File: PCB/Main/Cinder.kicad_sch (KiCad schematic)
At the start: 22 parts, among them J1 Heater -, J2 Heater +, J3 Fan +, J4 Fan -, Q1 IPD33CN10N G, Q2 IPD33CN10N G, SW1 SW_Push, SW2 SW_Push, SW3 SW_Push, SW9 EC11E09244BS, U1 RP2040-ZERO, U2 HS96L03W2C03, U3 XT60PW-F_C428722, U4 K7805-500R3_C909662

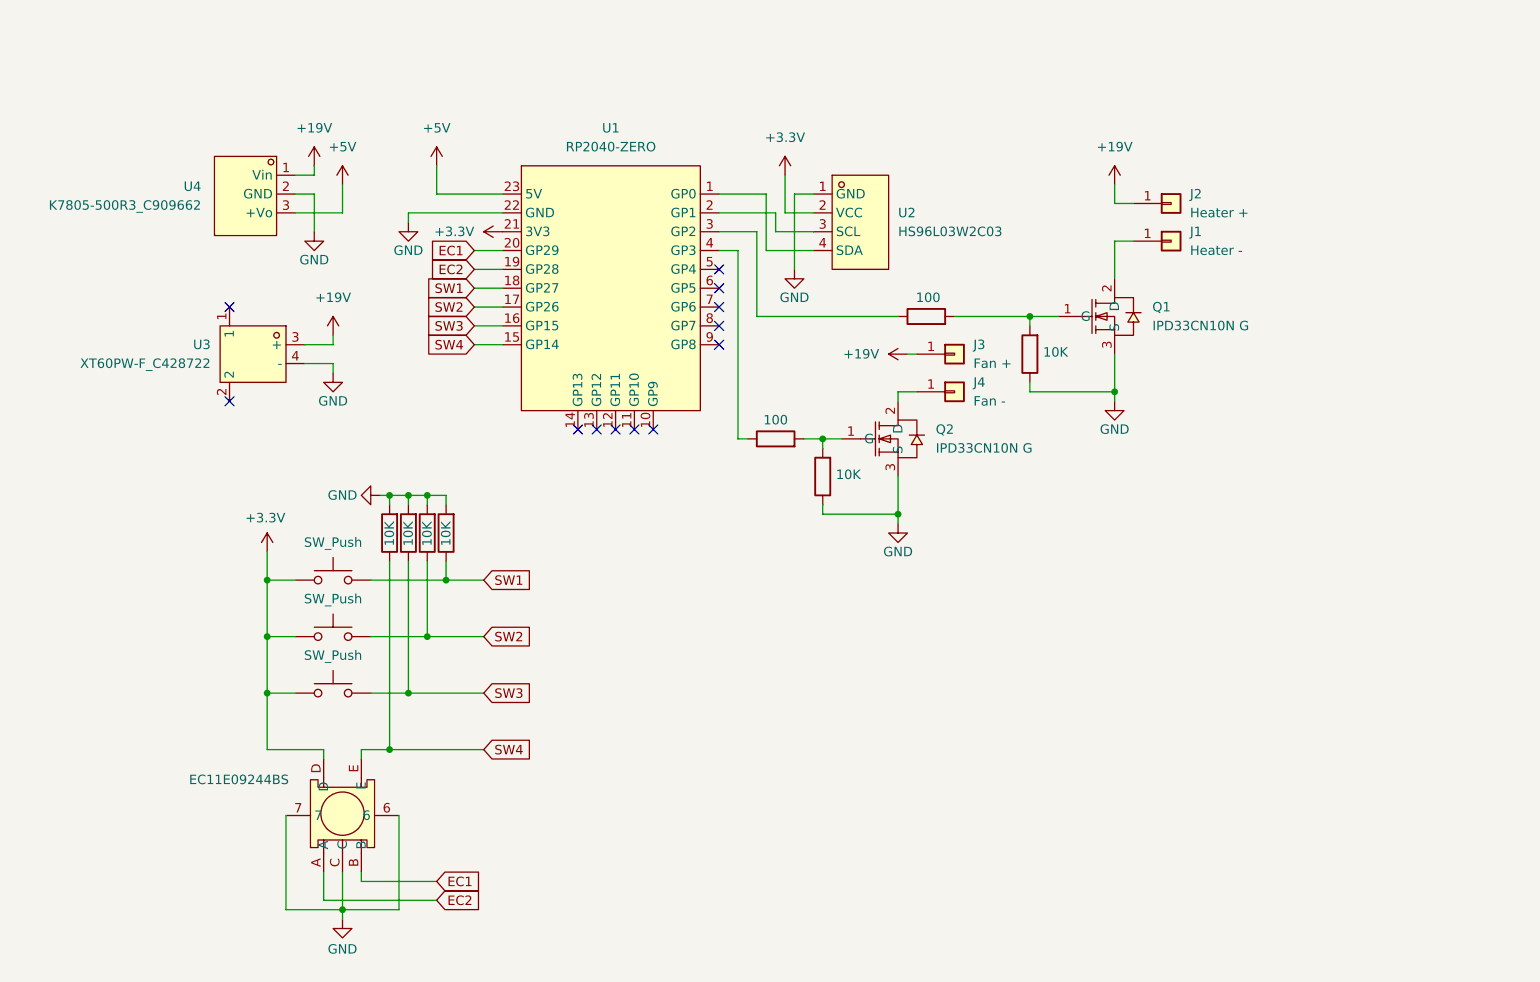
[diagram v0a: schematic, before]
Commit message: Update
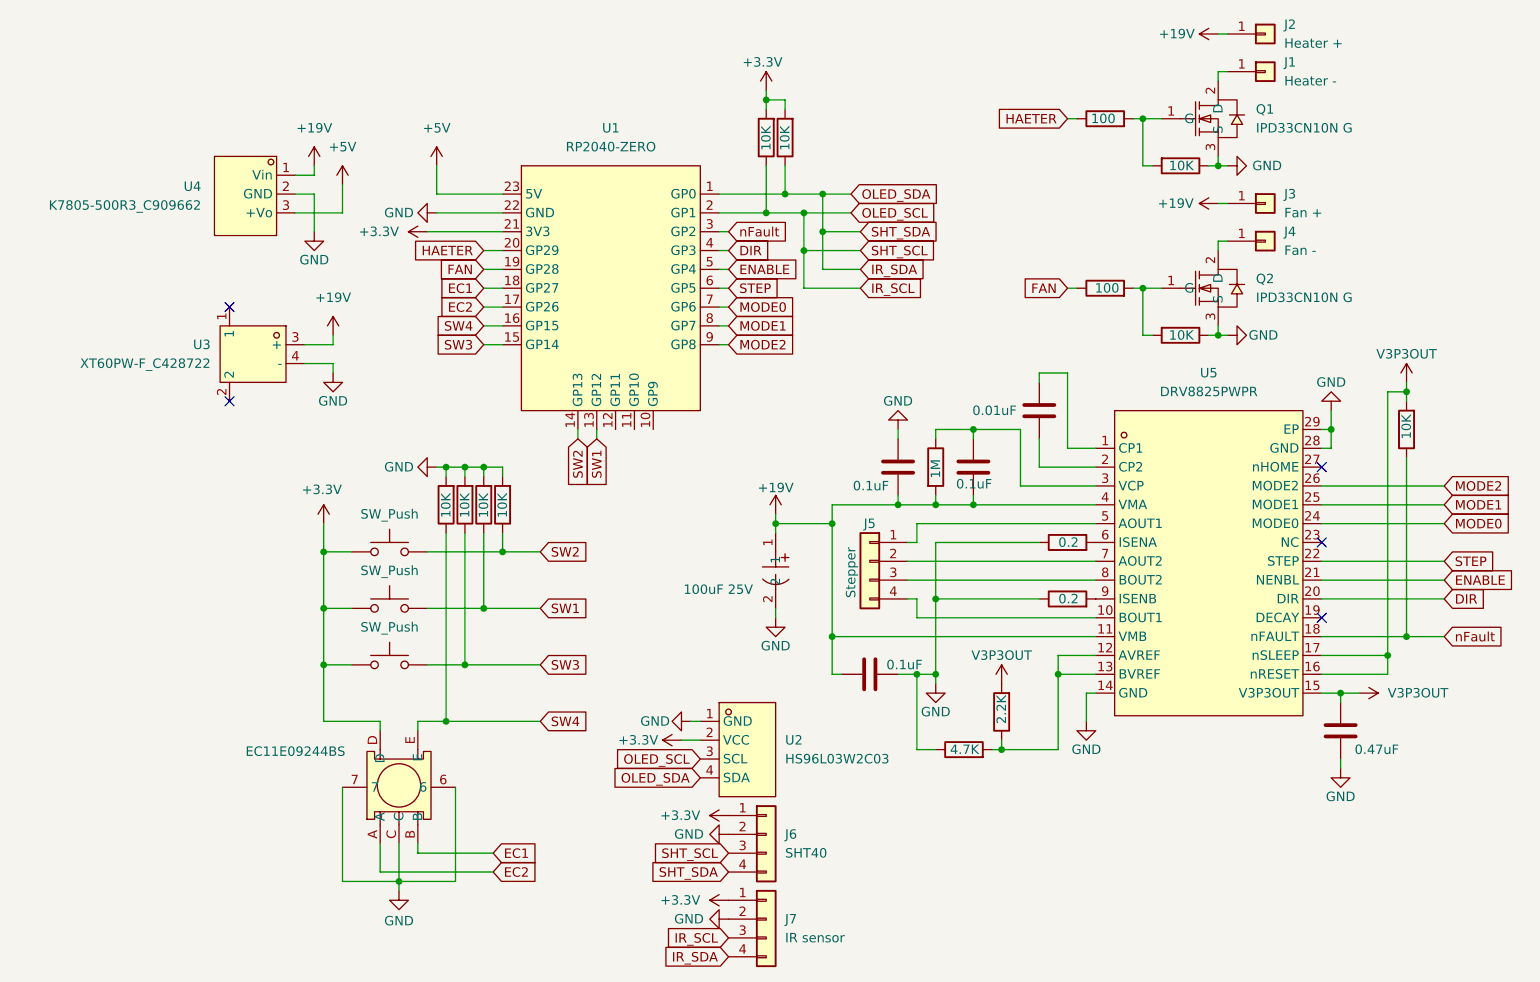
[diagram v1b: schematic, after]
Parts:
- added C1: 0.01uF, Capacitor_SMD:C_1206_3216Metric_Pad1.33x1.80mm_HandSolder, symbol Device:C
- added C2, C3, C4: 0.1uF, Capacitor_SMD:C_1206_3216Metric_Pad1.33x1.80mm_HandSolder, symbol Device:C
- added C5: 0.47uF, Capacitor_SMD:C_1206_3216Metric_Pad1.33x1.80mm_HandSolder, symbol Device:C
- added J5: Stepper, Connector_PinHeader_2.54mm:PinHeader_1x04_P2.54mm_Vertical, symbol Connector_Generic:Conn_01x04
- added J6: SHT40, Connector_PinHeader_2.54mm:PinHeader_1x04_P2.54mm_Vertical, symbol Connector_Generic:Conn_01x04
- added J7: IR sensor, Connector_PinHeader_2.54mm:PinHeader_1x04_P2.54mm_Vertical, symbol Connector_Generic:Conn_01x04
- added R10, R11: 0.2, Resistor_SMD:R_1206_3216Metric_Pad1.30x1.75mm_HandSolder, symbol Device:R
- added R12: 2.2K, Resistor_SMD:R_1206_3216Metric_Pad1.30x1.75mm_HandSolder, symbol Device:R
- added R13: 4.7K, Resistor_SMD:R_1206_3216Metric_Pad1.30x1.75mm_HandSolder, symbol Device:R
- added R15, R16, R17: 10K, Resistor_SMD:R_1206_3216Metric_Pad1.30x1.75mm_HandSolder, symbol Device:R
- added R9: 1M, Resistor_SMD:R_1206_3216Metric_Pad1.30x1.75mm_HandSolder, symbol Device:R
- added U5: DRV8825PWPR, LCSC:HTSSOP-28_L9.7-W4.4-P0.65-LS6.4-BL-EP5.5, symbol LCSC:DRV8825PWPR
- added U6: 100uF 25V, LCSC:CAP-SMD_BD6.3-L6.6-W6.6-LS7.2-FD-1, symbol LCSC:RVT1E101M0607100UF25V
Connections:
- net +19V: now also C2.2, C3.1, C4.1, R9.2, U5.11 (VMB), U5.4 (VMA), U6.1
- net +3.3V: now also J6.1 (Pin_1), J7.1 (Pin_1), R16.2, R17.2
- net EC1: now also U1.18 (GP27); no longer U1.20 (GP29)
- net EC2: now also U1.17 (GP26); no longer U1.19 (GP28)
- net GND: now also C3.2, C4.2, C5.2, J6.2 (Pin_2), J7.2 (Pin_2), R10.1, R11.1, R13.1, U5.14 (GND), U5.28 (GND), U5.29 (EP), U6.2
- net SW1: now also R6.1, SW1.2, U1.13 (GP12); no longer R5.1, SW2.2, U1.18 (GP27)
- net SW2: now also R5.1, SW2.2, U1.14 (GP13); no longer R6.1, SW1.2, U1.17 (GP26)
- net SW3: now also U1.15 (GP14); no longer U1.16 (GP15)
- net SW4: now also U1.16 (GP15); no longer U1.15 (GP14)
- net IR_SCL: now reaches U1.2 (GP1), U2.3 (SCL)
- net IR_SCL: now also J6.3 (Pin_3), J7.3 (Pin_3), R16.1
- net IR_SDA: now reaches U1.1 (GP0), U2.4 (SDA)
- net IR_SDA: now also J6.4 (Pin_4), J7.4 (Pin_4), R17.1
- net HAETER: now reaches R1.1
- net HAETER: now also U1.20 (GP29); no longer U1.3 (GP2)
- net DIR: now reaches U1.4 (GP3)
- net DIR: now also U5.20 (DIR); no longer R2.1
- net ENABLE: now reaches U1.5 (GP4)
- net ENABLE: now also U5.21 (NENBL)
- net STEP: now reaches U1.6 (GP5)
- net STEP: now also U5.22 (STEP)
- net MODE0: now reaches U1.7 (GP6)
- net MODE0: now also U5.24 (MODE0)
- net MODE1: now reaches U1.8 (GP7)
- net MODE1: now also U5.25 (MODE1)
- net MODE2: now reaches U1.9 (GP8)
- net MODE2: now also U5.26 (MODE2)
- new net: C1.1, U5.1 (CP1)
- new net: J5.4 (Pin_4), U5.10 (BOUT1)
- new net: R12.1, R13.2, U5.12 (AVREF), U5.13 (BVREF)
- new net: C1.2, U5.2 (CP2)
- new net: C2.1, R9.1, U5.3 (VCP)
- new net: J5.1 (Pin_1), U5.5 (AOUT1)
- new net: R10.2, U5.6 (ISENA)
- new net: J5.2 (Pin_2), U5.7 (AOUT2)
- new net: J5.3 (Pin_3), U5.8 (BOUT2)
- new net: R11.2, U5.9 (ISENB)
- new net FAN: R2.1, U1.19 (GP28)
- new net V3P3OUT: C5.1, R12.2, R15.2, U5.15 (V3P3OUT), U5.16 (nRESET), U5.17 (nSLEEP)
- new net nFault: R15.1, U1.3 (GP2), U5.18 (nFAULT)
- no-connect marks 12 -> 5
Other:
- moved on the sheet: J1, J2, J3, J4, Q1, Q2, U2
